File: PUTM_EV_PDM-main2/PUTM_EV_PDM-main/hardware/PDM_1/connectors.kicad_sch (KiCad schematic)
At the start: 3 parts, among them J3 UPT-08-03.0-01-L-V, J4 UPT-08-03.0-01-L-V, J5 UPT-02-01-01-X-RA

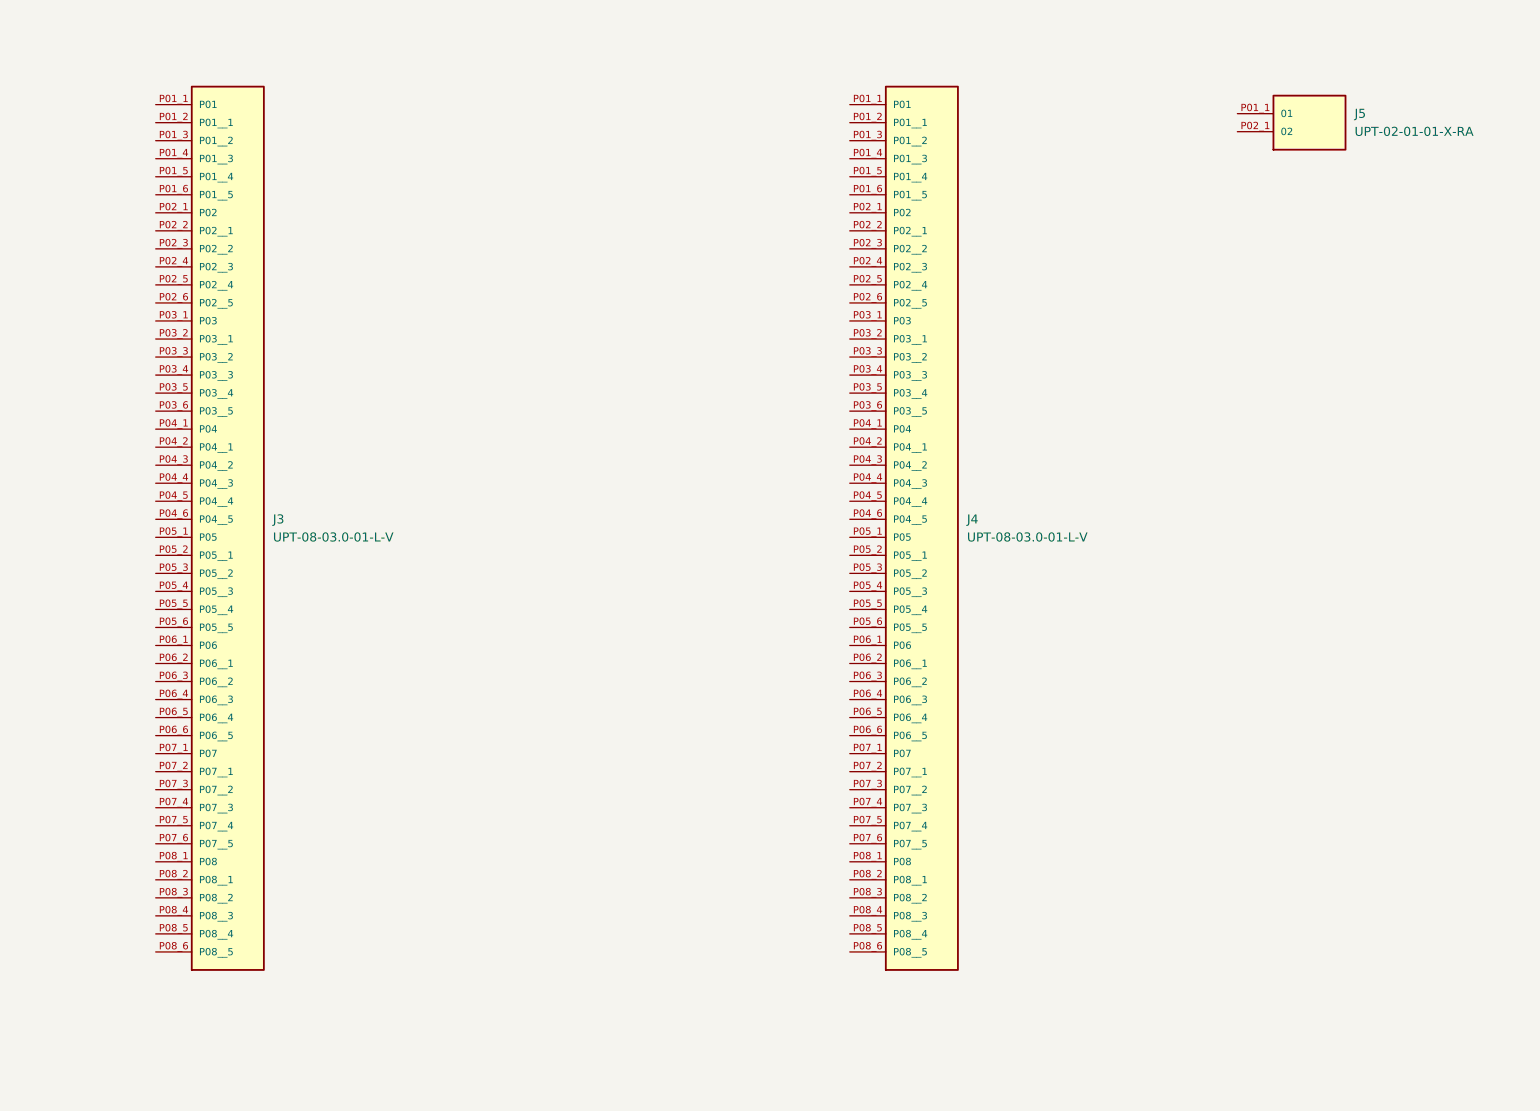
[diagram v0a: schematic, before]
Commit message: piny na płytce
Dodano ułożenie pinów na płytce
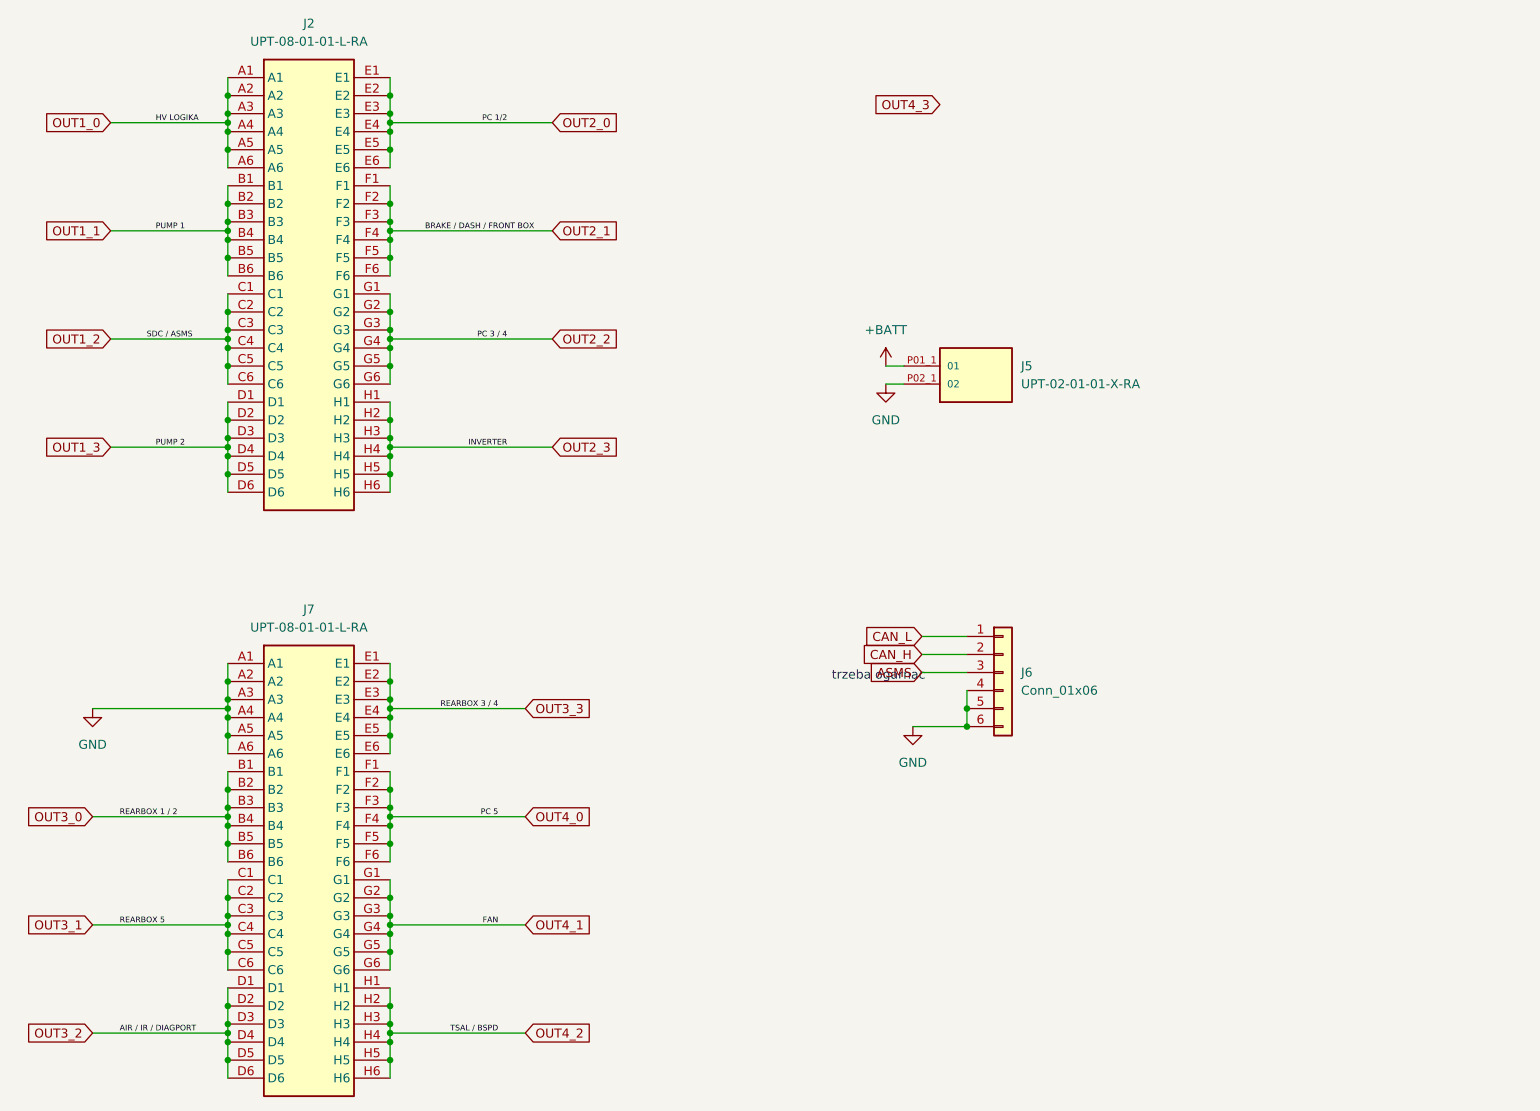
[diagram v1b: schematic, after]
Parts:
- removed J3, J4: UPT-08-03.0-01-L-V, UPT-08-03.0-01-L-V:SAMTEC_UPT-08-03.0-01-L-V, symbol 8pin:UPT-08-03.0-01-L-V
- added J2, J7: UPT-08-01-01-L-RA, UPT080101LRA, symbol 8pin_good:UPT-08-01-01-L-RA
- added J6: Conn_01x06, Connector_IDC:IDC-Header_2x03_P2.54mm_Vertical, symbol Connector_Generic:Conn_01x06
- J5: footprint UPT-02-01-01-X-RA:SAMTEC_UPT-02-01-01-X-RA -> 2pin:SAMTEC_UPT-02-01-01-X-RA
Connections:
- net +BATT: now reaches J5.P01_1 (01)
- net GND: now reaches J5.P02_1 (02)
- net GND: now also J6.4 (Pin_4), J6.5 (Pin_5), J6.6 (Pin_6), J7.A1, J7.A2, J7.A3, J7.A4, J7.A5, J7.A6
- new net ASMS: J6.3 (Pin_3)
- new net CAN_H: J6.2 (Pin_2)
- new net CAN_L: J6.1 (Pin_1)
- new net OUT1_0: J2.A1, J2.A2, J2.A3, J2.A4, J2.A5, J2.A6
- new net OUT1_1: J2.B1, J2.B2, J2.B3, J2.B4, J2.B5, J2.B6
- new net OUT1_2: J2.C1, J2.C2, J2.C3, J2.C4, J2.C5, J2.C6
- new net OUT1_3: J2.D1, J2.D2, J2.D3, J2.D4, J2.D5, J2.D6
- new net OUT2_0: J2.E1, J2.E2, J2.E3, J2.E4, J2.E5, J2.E6
- new net OUT2_1: J2.F1, J2.F2, J2.F3, J2.F4, J2.F5, J2.F6
- new net OUT2_2: J2.G1, J2.G2, J2.G3, J2.G4, J2.G5, J2.G6
- new net OUT2_3: J2.H1, J2.H2, J2.H3, J2.H4, J2.H5, J2.H6
- new net OUT3_0: J7.B1, J7.B2, J7.B3, J7.B4, J7.B5, J7.B6
- new net OUT3_1: J7.C1, J7.C2, J7.C3, J7.C4, J7.C5, J7.C6
- new net OUT3_2: J7.D1, J7.D2, J7.D3, J7.D4, J7.D5, J7.D6
- new net OUT3_3: J7.E1, J7.E2, J7.E3, J7.E4, J7.E5, J7.E6
- new net OUT4_0: J7.F1, J7.F2, J7.F3, J7.F4, J7.F5, J7.F6
- new net OUT4_1: J7.G1, J7.G2, J7.G3, J7.G4, J7.G5, J7.G6
- new net OUT4_2: J7.H1, J7.H2, J7.H3, J7.H4, J7.H5, J7.H6
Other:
- note added: "trzeba ogarnac"
- moved on the sheet: J5
